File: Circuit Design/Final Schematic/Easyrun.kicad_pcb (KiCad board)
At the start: 2 copper layers, 100 x 92.5 mm, 78 parts, among them U1 ESP32-WROOM-32

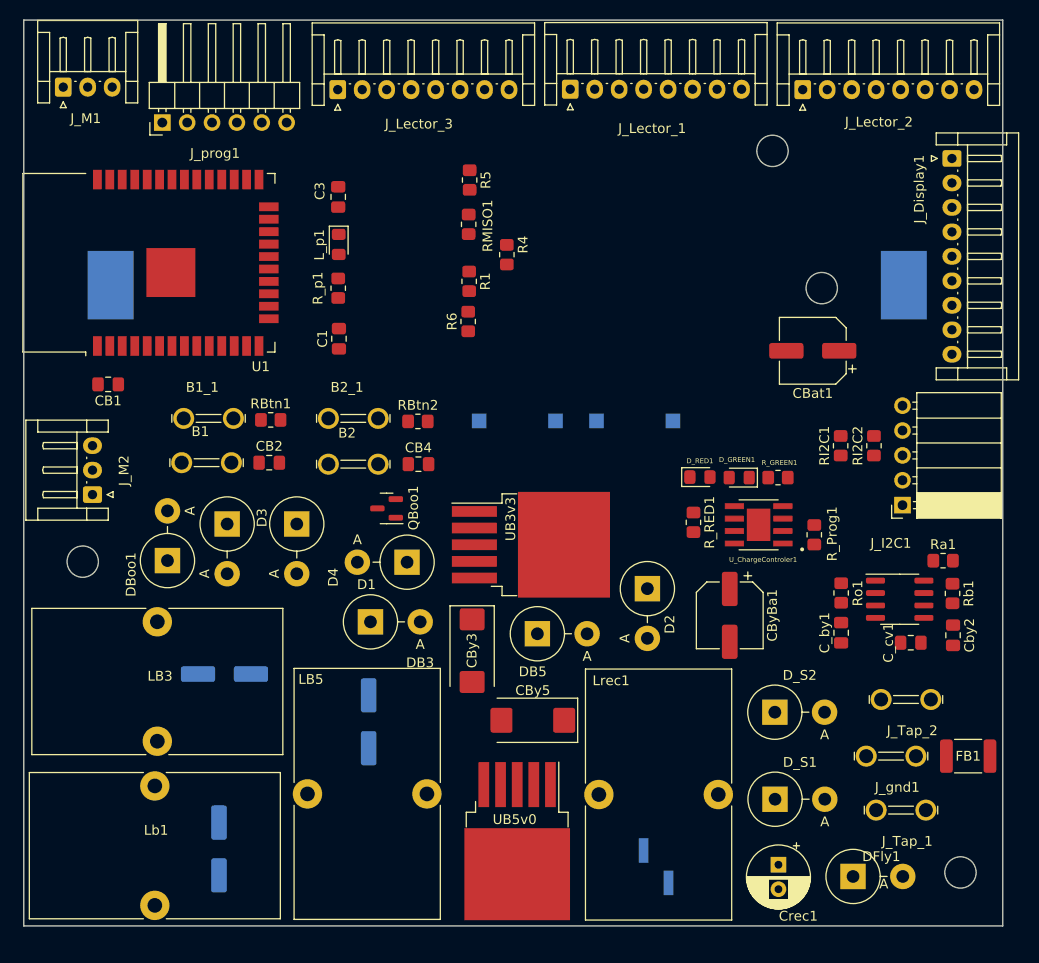
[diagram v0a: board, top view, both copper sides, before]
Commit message: PCB almost ready
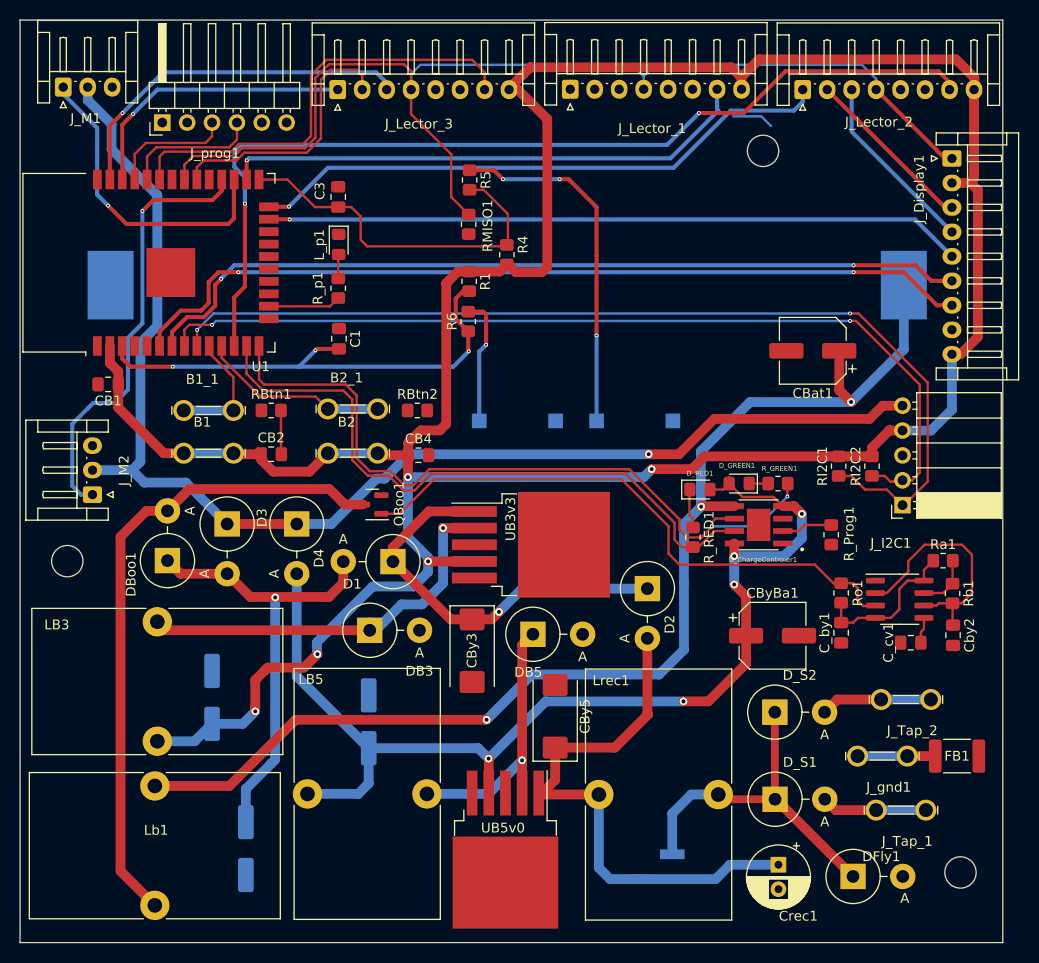
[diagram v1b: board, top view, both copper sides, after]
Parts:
- moved CByBa1 4.84 mm to (148.4, 103.3), turned to 0 degrees
- moved C_b1 2.75 mm to (94.6, 125.0)
- moved CB3 2.70 mm to (91.2, 109.6), turned to 90 degrees
- moved CBy5 2.32 mm to (126.2, 111.5), turned to 90 degrees
- moved RI2C1 2.09 mm to (155.2, 86.0)
- moved RI2C2 2.09 mm to (158.6, 86.0)
- moved R_Prog1 1.73 mm to (154.4, 93.0)
- moved REF** 1.58 mm to (76.4, 95.7)
- moved QBoo1 1.53 mm to (107.5, 89.9)
- moved R_RED1 1.52 mm to (140.3, 93.2)
- moved UB5v0 1.48 mm to (121.2, 125.1)
- moved D1 1.44 mm to (109.7, 95.7)
- moved D_RED1 1.27 mm to (141.0, 88.3)
- moved FB1 1.14 mm to (167.3, 115.6)
- moved RBtn2 1.12 mm to (112.2, 80.3)
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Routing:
- net +3V3: track 0.00 -> 296.0 mm, vias 0 -> 5
- net +5V: track 0.00 -> 133.2 mm, vias 0 -> 1
- net /PowerModule/Battery Charge/Vo_bat: track 0.00 -> 121.6 mm, vias 0 -> 3
- net /MISO: track 0.00 -> 114.0 mm
- net /PowerModule/Buck5v0: track 0.00 -> 111.6 mm, vias 0 -> 5
- net /I2C2: track 0.00 -> 101.3 mm, vias 0 -> 2
- net /Rst_2: track 0.00 -> 98.5 mm, vias 0 -> 2
- net /I2C1: track 0.00 -> 94.3 mm, vias 0 -> 2
- net /CS_Display: track 0.00 -> 87.6 mm, vias 0 -> 2
- net /Rst_D: track 0.00 -> 85.9 mm, vias 0 -> 2
- net STDBY: track 0.00 -> 75.8 mm, vias 0 -> 2
- net /D/C: track 0.00 -> 71.4 mm, vias 0 -> 1
- net CHRG: track 0.00 -> 66.8 mm
- net Net-(DBoo1-Pad2): track 0.00 -> 66.5 mm
- net /CS_Lector2: track 0.00 -> 60.2 mm, vias 0 -> 1
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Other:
- board size 100 x 92.5 mm -> 100.4 x 94.2 mm
